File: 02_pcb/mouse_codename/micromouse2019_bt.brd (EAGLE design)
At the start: 13 x 17.8 mm, 2 parts, among them U1 SPBT2632C2A.AT2

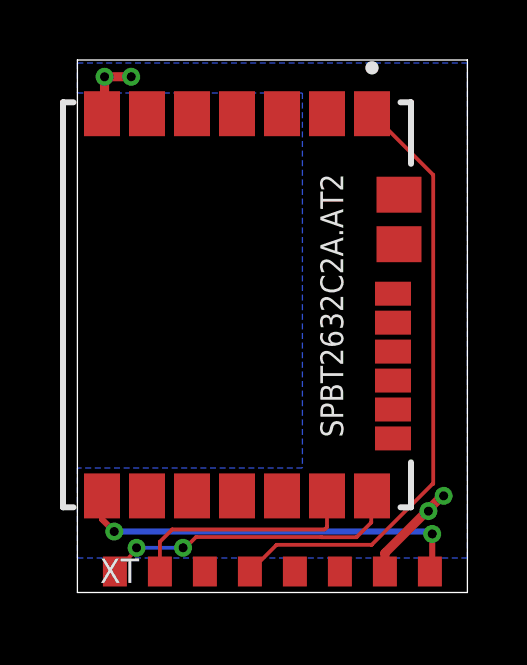
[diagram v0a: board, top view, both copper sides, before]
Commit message: minor board updates
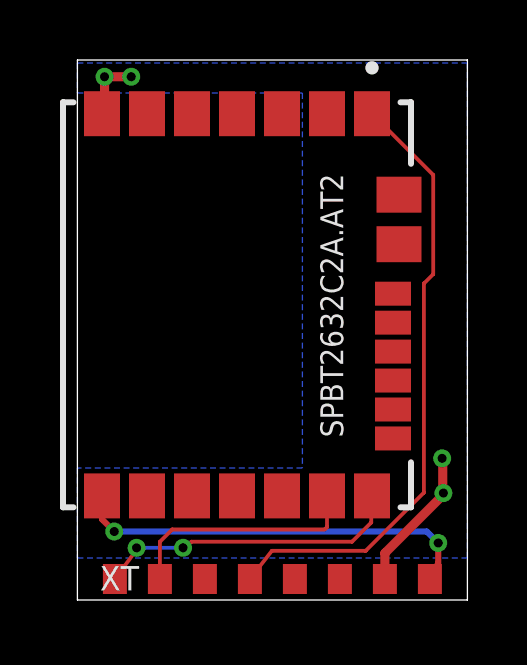
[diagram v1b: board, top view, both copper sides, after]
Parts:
- moved PORT1 0.25 mm to (7.50, 1.80)
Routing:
- net GND: track 5.53 -> 6.99 mm
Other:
- board size 13 x 17.8 mm -> 13 x 18 mm
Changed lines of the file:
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@@
 <drawing>
 <settings>
-<setting alwaysvectorfont="no"/>
+<setting alwaysvectorfont="yes"/>
 <setting verticaltext="up"/>
 </settings>
-<grid distance="3.93700787" unitdist="mil" unit="mil" style="lines" multiple="1" display="yes" altdistance="1" altunitdist="mil" altunit="mil"/>
+<grid distance="1.96850394" unitdist="mil" unit="mil" style="lines" multiple="1" display="yes" altdistance="1" altunitdist="mil" altunit="mil"/>
 <layers>
 <layer number="1" name="Top" color="4" fill="1" visible="yes" active="yes"/>
@@
 <layer number="27" name="tValues" color="7" fill="1" visible="yes" active="yes"/>
 <layer number="28" name="bValues" color="7" fill="1" visible="yes" active="yes"/>
-<layer number="29" name="tStop" color="7" fill="3" visible="no" active="yes"/>
+<layer number="29" name="tStop" color="7" fill="3" visible="yes" active="yes"/>
 <layer number="30" name="bStop" color="7" fill="6" visible="no" active="yes"/>
 <layer number="31" name="tCream" color="7" fill="4" visible="no" active="yes"/>
@@
 <board>
 <plain>
-<wire x1="1" y1="1.35" x2="14" y2="1.35" width="0" layer="20"/>
-<wire x1="14" y1="1.35" x2="14" y2="19.1" width="0" layer="20"/>
+<wire x1="1" y1="1.1" x2="14" y2="1.1" width="0" layer="20"/>
+<wire x1="14" y1="1.1" x2="14" y2="19.1" width="0" layer="20"/>
 <wire x1="14" y1="19.1" x2="1" y2="19.1" width="0" layer="20"/>
-<wire x1="1" y1="19.1" x2="1" y2="1.35" width="0" layer="20"/>
+<wire x1="1" y1="19.1" x2="1" y2="1.1" width="0" layer="20"/>
 <dimension x1="14" y1="19" x2="1" y2="19" x3="7.5" y3="25" textsize="1.778" layer="47"/>
 <dimension x1="14" y1="1.35" x2="14" y2="19" x3="22" y3="10.175" textsize="1.778" layer="47"/>
@@
 </autorouter>
 <elements>
-<element name="PORT1" library="0-micromouse2019" package="BT_PORT_MODULE" package3d_urn="urn:adsk.eagle:package:9190656/1" value="PORT_BT_MODULE" x="7.5" y="2.05" smashed="yes">
-<attribute name="VALUE" x="1.75" y="0.518334375" size="0.7" layer="27"/>
+<element name="PORT1" library="0-micromouse2019" package="BT_PORT_MODULE" package3d_urn="urn:adsk.eagle:package:9190656/1" value="PORT_BT_MODULE" x="7.5" y="1.8" smashed="yes">
+<attribute name="VALUE" x="1.75" y="0.268334375" size="0.7" layer="27"/>
 </element>
 <element name="U1" library="0-micromouse2019" package="XCVR_SPBT2632C2A.AT2" value="SPBT2632C2A.AT2" x="6.32" y="10.94" smashed="yes" rot="R270">
@@
 <contactref element="PORT1" pad="P15"/>
 <via x="2.2278" y="3.3828" extent="1-16" drill="0.3" diameter="0.6"/>
-<wire x1="12.75" y1="2.05" x2="12.843" y2="2.143" width="0.254" layer="1"/>
 <wire x1="1.82" y1="4.57" x2="1.82" y2="3.7906" width="0.2032" layer="1"/>
 <wire x1="1.82" y1="3.7906" x2="2.2278" y2="3.3828" width="0.2032" layer="1"/>
-<wire x1="2.2278" y1="3.3828" x2="12.7462" y2="3.3828" width="0.2032" layer="16"/>
-<wire x1="12.7462" y1="3.3828" x2="12.827" y2="3.302" width="0.2032" layer="16"/>
-<via x="12.827" y="3.302" extent="1-16" drill="0.3" diameter="0.6"/>
-<wire x1="12.827" y1="3.302" x2="12.827" y2="2.159" width="0.2032" layer="1"/>
-<wire x1="12.827" y1="2.159" x2="12.843" y2="2.143" width="0.2032" layer="1"/>
+<wire x1="2.2278" y1="3.3828" x2="12.6462" y2="3.3828" width="0.2032" layer="16"/>
+<wire x1="12.6462" y1="3.3828" x2="13.027" y2="3.002" width="0.2032" layer="16"/>
+<via x="13.027" y="3.002" extent="1-16" drill="0.3" diameter="0.6"/>
+<wire x1="13.027" y1="3.002" x2="13.027" y2="2.327" width="0.2032" layer="1"/>
+<wire x1="12.75" y1="1.8" x2="13.027" y2="2.327" width="0.2032" layer="1"/>
 </signal>
 <signal name="GND">
@@
 <contactref element="PORT1" pad="P14"/>
 <wire x1="13.178" y1="4.59" x2="11.25" y2="2.662" width="0.3048" layer="1"/>
-<wire x1="11.25" y1="2.662" x2="11.25" y2="2.05" width="0.3048" layer="1"/>
-<polygon width="0.1524" layer="16">
+<wire x1="11.25" y1="2.662" x2="11.25" y2="1.8" width="0.3048" layer="1"/>
+<polygon width="0.1524" layer="16" isolate="0.254">
 <vertex x="1" y="19"/>
 <vertex x="1" y="18"/>
@@
 <vertex x="14" y="19"/>
 </polygon>
-<via x="13.208" y="4.572" extent="1-16" drill="0.3" diameter="0.6"/>
-<wire x1="13.208" y1="4.572" x2="13.196" y2="4.572" width="0.1524" layer="1"/>
-<wire x1="13.196" y1="4.572" x2="13.178" y2="4.59" width="0.1524" layer="1"/>
-<via x="12.7" y="4.064" extent="1-16" drill="0.3" diameter="0.6"/>
+<via x="13.158" y="5.822" extent="1-16" drill="0.3" diameter="0.6"/>
+<wire x1="13.158" y1="5.822" x2="13.178" y2="5.802" width="0.1524" layer="1"/>
+<wire x1="13.178" y1="5.802" x2="13.178" y2="4.59" width="0.3048" layer="1"/>
+<via x="13.2" y="4.664" extent="1-16" drill="0.3" diameter="0.6"/>
 <via x="1.905" y="18.542" extent="1-16" drill="0.3" diameter="0.6"/>
 <via x="2.794" y="18.542" extent="1-16" drill="0.3" diameter="0.6"/>
@@
 <wire x1="10.82" y1="4.57" x2="10.795" y2="4.545" width="0.127" layer="1"/>
 <wire x1="10.795" y1="4.545" x2="10.795" y2="3.683" width="0.127" layer="1"/>
-<wire x1="9.1357875" y1="3.193" x2="9.1297875" y2="3.199" width="0.127" layer="1"/>
-<wire x1="9.1297875" y1="3.199" x2="4.953" y2="3.199" width="0.127" layer="1"/>
-<wire x1="10.795" y1="3.683" x2="10.305" y2="3.193" width="0.127" layer="1"/>
-<wire x1="10.305" y1="3.193" x2="9.1357875" y2="3.193" width="0.127" layer="1"/>
-<wire x1="4.953" y1="3.199" x2="4.5215" y2="2.7675" width="0.127" layer="1"/>
-<wire x1="4.5215" y1="2.7675" x2="4.5223" y2="2.8402625" width="0.127" layer="1"/>
+<wire x1="10.155" y1="3.043" x2="4.797" y2="3.043" width="0.127" layer="1"/>
+<wire x1="10.795" y1="3.683" x2="10.155" y2="3.043" width="0.127" layer="1"/>
 <via x="4.5223" y="2.8402625" extent="1-16" drill="0.3" diameter="0.6"/>
 <wire x1="4.5223" y1="2.8402625" x2="2.9729" y2="2.8388625" width="0.127" layer="16"/>
 <via x="2.9729" y="2.8388625" extent="1-16" drill="0.3" diameter="0.6"/>
 <wire x1="2.9729" y1="2.8388625" x2="2.9675" y2="2.7675" width="0.127" layer="1"/>
-<wire x1="2.9675" y1="2.7675" x2="2.25" y2="2.05" width="0.127" layer="1"/>
+<wire x1="2.9675" y1="2.7675" x2="2.25" y2="1.8" width="0.127" layer="1"/>
+<wire x1="4.5223" y1="2.8402625" x2="4.5942625" y2="2.8402625" width="0.127" layer="1"/>
+<wire x1="4.5942625" y1="2.8402625" x2="4.797" y2="3.043" width="0.127" layer="1"/>
 </signal>
 <signal name="STATUS">
 <contactref element="U1" pad="1"/>
 <contactref element="PORT1" pad="P11"/>
-<wire x1="12.84040625" y1="4.971" x2="12.8605" y2="4.971" width="0.127" layer="1"/>
-<wire x1="10.80840625" y1="2.939" x2="12.84040625" y2="4.971" width="0.127" layer="1"/>
-<wire x1="12.8605" y1="4.971" x2="12.8605" y2="15.2695" width="0.127" layer="1"/>
-<wire x1="12.8605" y1="15.2695" x2="10.82" y2="17.31" width="0.127" layer="1"/>
-<wire x1="6.75" y1="2.05" x2="7.639" y2="2.939" width="0.127" layer="1"/>
-<wire x1="7.639" y1="2.939" x2="10.80840625" y2="2.939" width="0.127" layer="1"/>
+<wire x1="10.60840625" y1="2.739" x2="12.55" y2="4.68059375" width="0.127" layer="1"/>
+<wire x1="10.82" y1="17.31" x2="12.8605" y2="15.2695" width="0.127" layer="1"/>
+<wire x1="6.75" y1="1.8" x2="7.482896875" y2="2.739" width="0.127" layer="1"/>
+<wire x1="7.482896875" y1="2.739" x2="10.60840625" y2="2.739" width="0.127" layer="1"/>
+<wire x1="12.8605" y1="15.2695" x2="12.8605" y2="11.9605" width="0.127" layer="1"/>
+<wire x1="12.8605" y1="11.9605" x2="12.55" y2="11.65" width="0.127" layer="1"/>
+<wire x1="12.55" y1="11.65" x2="12.55" y2="4.68059375" width="0.127" layer="1"/>
 </signal>
 <signal name="BT_RX">
@@
 <contactref element="PORT1" pad="P9"/>
 <wire x1="4.161" y1="3.453" x2="3.75" y2="3.042" width="0.127" layer="1"/>
-<wire x1="3.75" y1="3.042" x2="3.75" y2="2.05" width="0.127" layer="1"/>
+<wire x1="3.75" y1="3.042" x2="3.75" y2="1.8" width="0.127" layer="1"/>
 </signal>
 </signals>
